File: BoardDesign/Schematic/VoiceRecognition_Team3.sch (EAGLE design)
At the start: 47 parts, among them J1 5.5x2.1mm Barrel, Q1 16MHz, X1 USB-A

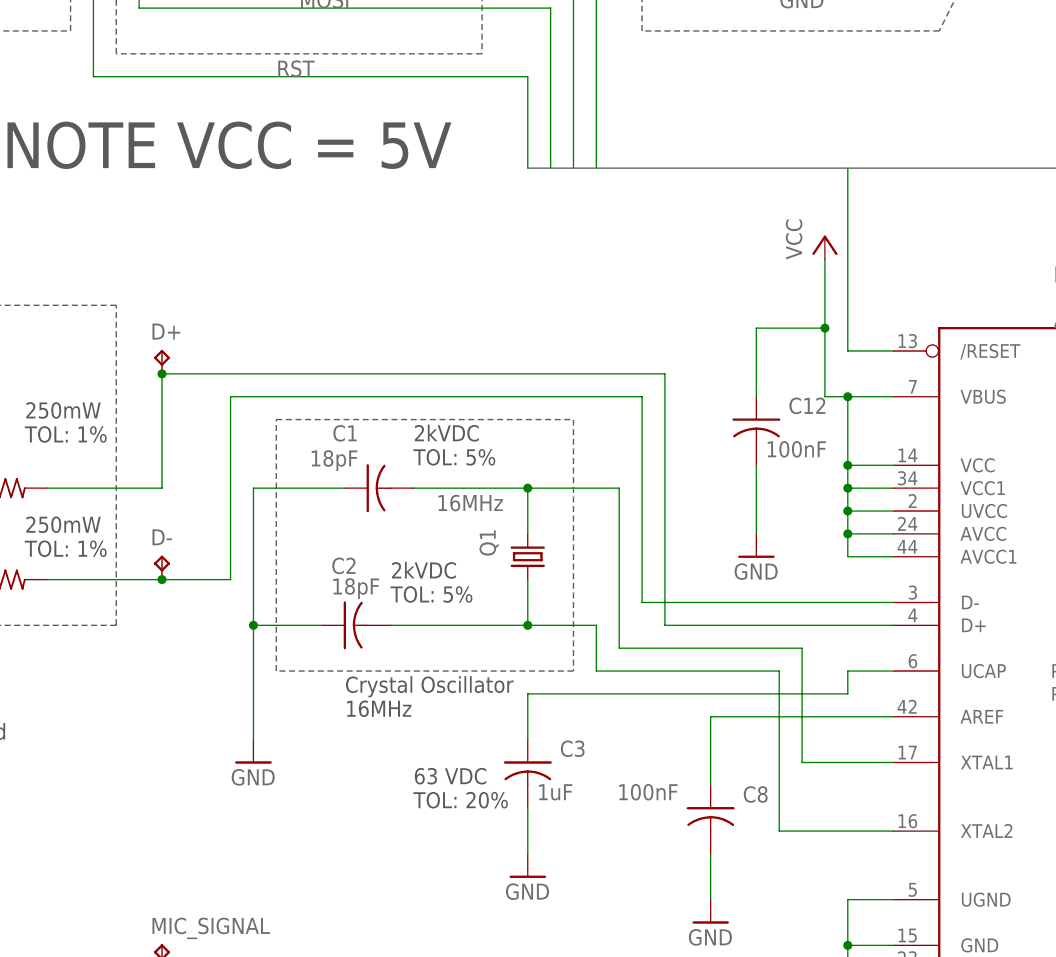
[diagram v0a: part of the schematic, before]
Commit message: Added a few changes to the board per andrew's suggestion
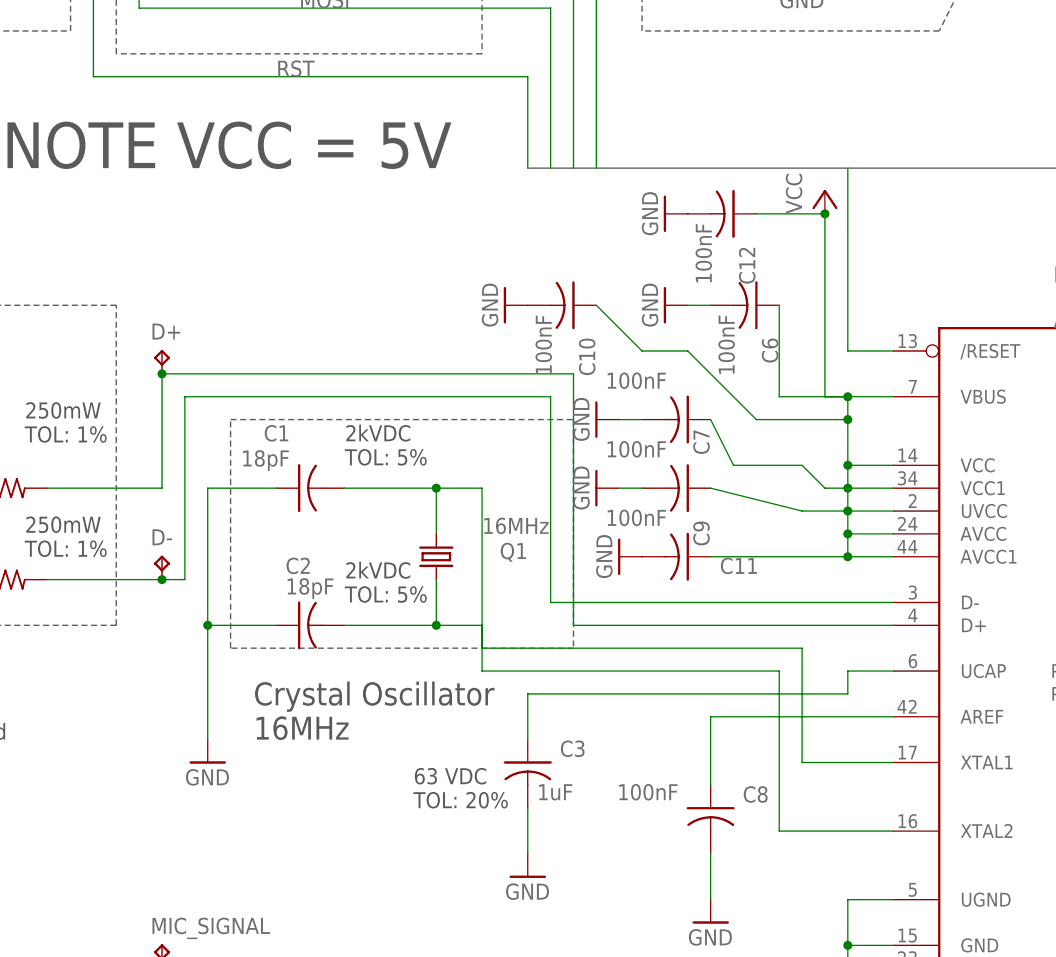
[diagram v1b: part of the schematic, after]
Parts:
- added C10, C11, C6, C7, C9: 100nF, rcl:C-USC1206
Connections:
- net GND: now also C10.2, C11.2, C6.2, C7.2, C9.2
- net VCC: now also C10.1, C11.1, C6.1, C7.1, C9.1
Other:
- moved on the sheet: C1, C12, C2, Q1
